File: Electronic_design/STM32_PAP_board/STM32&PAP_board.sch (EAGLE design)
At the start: 20 parts

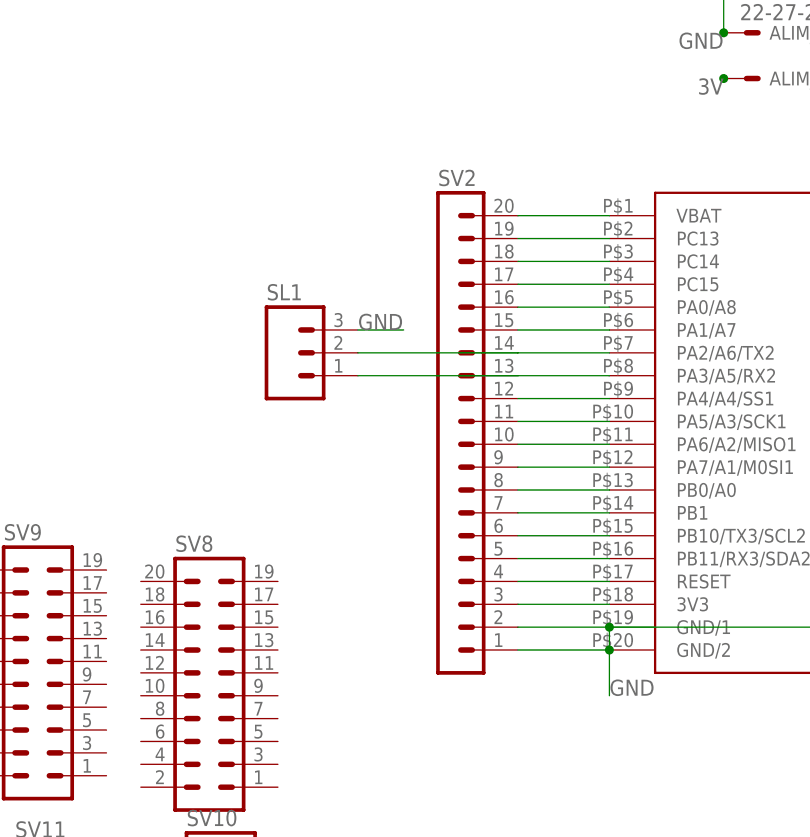
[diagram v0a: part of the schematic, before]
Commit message: ameliorations
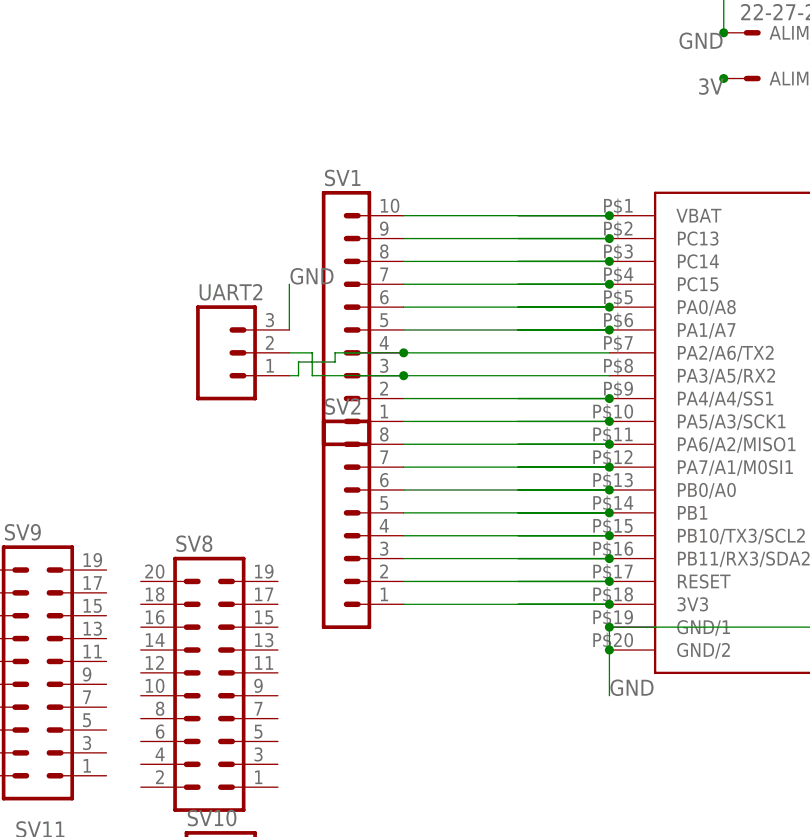
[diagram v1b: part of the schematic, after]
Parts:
- removed SL1: (no value), con-amp-quick:MA03
- added SV1: (no value), con-lstb:MA10-1
- added UART2: (no value), con-amp-quick:MA03
- SV2: device con-lstb:MA20-1 -> con-lstb:MA08-1
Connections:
- net GND: now also UART2.3; no longer SL1.3, SV2.1, SV2.2
- net N$10: now also SV2.8; no longer SV2.10
- net N$11: now also SV1.1; no longer SV2.11
- net N$12: now also SV1.2; no longer SV2.12
- net N$13: now also SV1.3, UART2.2; no longer SL1.1, SV2.13
- net N$14: now also SV1.4, UART2.1; no longer SL1.2, SV2.14
- net N$15: now also SV1.5; no longer SV2.15
- net N$16: now also SV1.6; no longer SV2.16
- net N$17: now also SV1.7; no longer SV2.17
- net N$18: now also SV1.8; no longer SV2.18
- net N$19: now also SV1.9; no longer SV2.19
- net N$20: now also SV1.10; no longer SV2.20
- net N$3: now also SV2.1; no longer SV2.3
- net N$4: now also SV2.2; no longer SV2.4
- net N$5: now also SV2.3; no longer SV2.5
- net N$6: now also SV2.4; no longer SV2.6
- net N$7: now also SV2.5; no longer SV2.7
- net N$8: now also SV2.6; no longer SV2.8
- net N$9: now also SV2.7; no longer SV2.9
